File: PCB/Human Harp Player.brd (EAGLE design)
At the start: 70 x 70 mm, 41 parts, among them J1 4UCON 20404, J3 Sparkfun: PRT-00553, J4 Sparkfun: PRT-00553, J5 Sparkfun: PRT-00553, J6 Sparkfun: PRT-00553, J7 ICSP, J8 Molex: 500075-1517, Q1 MMBT2222A, Q3 STD26P3LLH6, U1 DSPIC33EP512GM604-I/PT, U2 MIC5319-3.3YD5, U3 Sparkfun: PRT-00116, X1 ABM8-16.000MHZ-B2-T

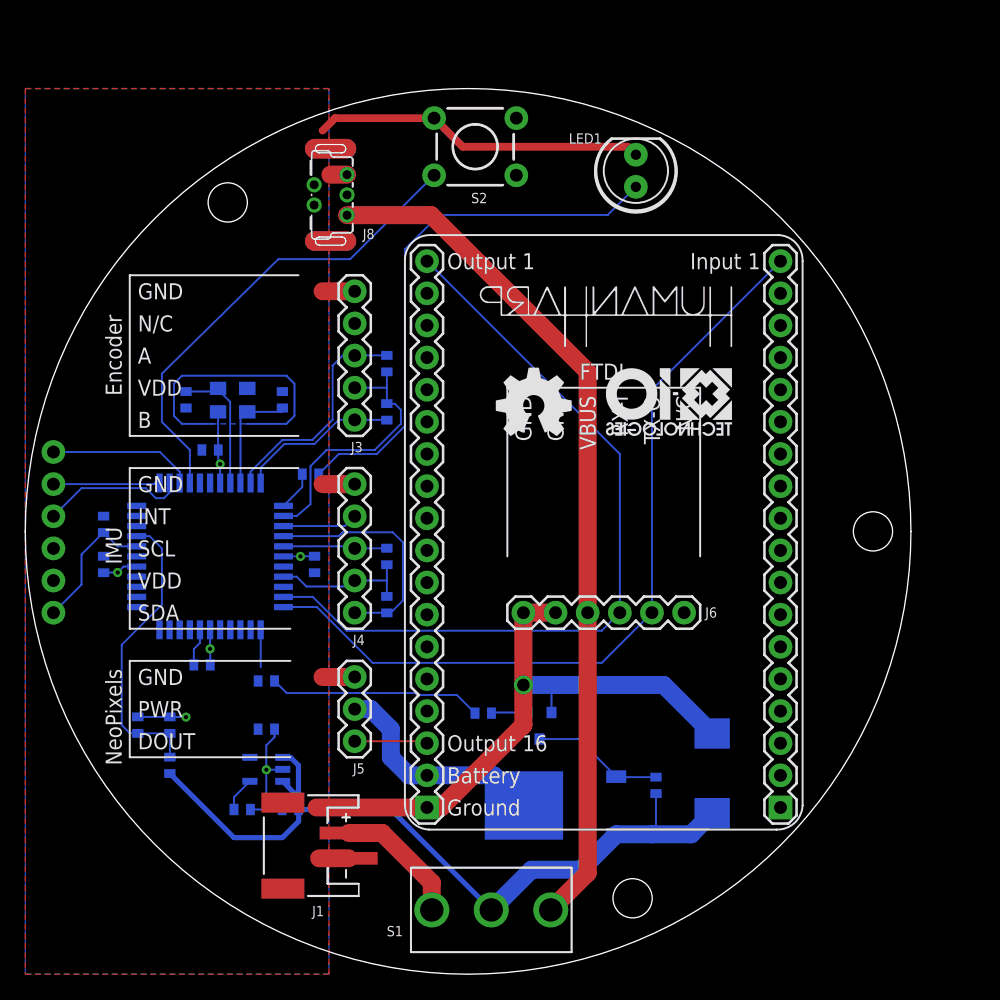
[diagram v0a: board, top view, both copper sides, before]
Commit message: Commit PCB Rev. 2
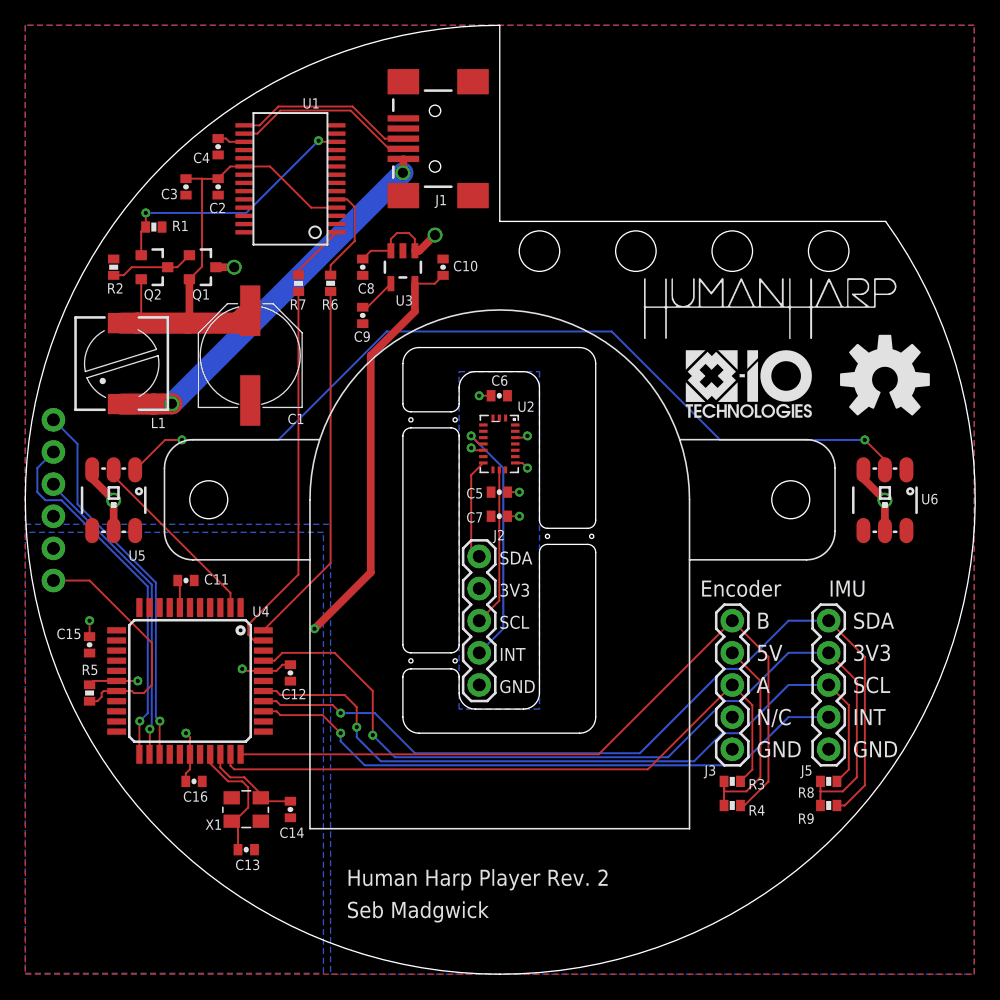
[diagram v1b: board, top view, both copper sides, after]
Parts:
- removed J6: Sparkfun: PRT-00553, SparkFun:1X06
- removed J7: ICSP, SparkFun-Connectors:1X06_NO_SILK
- removed J8: Molex: 500075-1517, x-io:500075-1517
- removed LED1: Sparkfun: COM-12903 (purple), SparkFun-LED:LED5MM
- removed Q3: STD26P3LLH6, transistor-fet:TO252
- removed R10: 10k, 0603, SparkFun:0402-RES
- removed R11: 15R, 0603, SparkFun:0402-RES
- removed S1: RS: 5MS1S102AM2QES, x-io:5MS1S102AM2QES
- removed S2: TE Connectivity: FSM4JAH, SparkFun-Electromechanical:TACTILE-PTH
- removed U$3: (no value), x-io:HUMAN_HARP_LOGO_20MM_BOTTOM
- added C12, C15, C16: 100n, 0603, SparkFun:0402-CAP
- added C13, C14: 22p, 0603, SparkFun:0402-CAP
- added J2: Unpopulated, SparkFun-Connectors:1X05
- added L1: 220u, 510mA, EATON-DRA73-221-R, rcl:PIS2816
- added LOGO1: OSHW-LOGOL, SparkFun-Aesthetics:OSHW-LOGO-L
- added Q2: IRLML6401PBF, SparkFun-DiscreteSemi:SOT23-3
- added U$2: (no value), x-io:HEDS-5600-A06
- added U4: DSPIC33EP512GM604-I/PT, x-io:TQFP44
- added U5, U6: WS2811, SparkFun-LED:LED-TRICOLOR-5050-IC
- C1: value 100n, 0603 -> 470u, 16V, Pansonic F; device SparkFun:0402-CAP -> rcl:PANASONIC_F
- C10, C8: value 100n, 0603 -> 10u, 0603
- C11: value 470u, 10V, Tant, Case E -> 10u, 0603; device rcl:SMC_E -> SparkFun:0402-CAP
- C5, C6: value 22p, 0603 -> 100n, 0603
- C9: value 10u, 0603 -> 100n, 0603
- J1: value 4UCON 20404 -> Sparkfun-PRT-00587; device x-io:JST-R/A -> SparkFun-Connectors:USB-MINIB
- J3: value Sparkfun: PRT-00553 -> Sparkfun: PRT-00116
- J4: value Sparkfun: PRT-00553 -> Unpopulated; device SparkFun-Connectors:1X05 -> SparkFun-Connectors:1X06_NO_SILK
- J5: value Sparkfun: PRT-00553 -> Sparkfun: PRT-00116; device SparkFun-Connectors:1X03 -> SparkFun-Connectors:1X05
- Q1: value MMBT2222A -> IRLML6401PBF
- R1, R6, R7: value 10k 0603 -> 4k7, 0603
- R2, R3, R4, R5, R8, R9: value 10k, 0603 -> 4k7, 0603
- U$1: device x-io:X-IO_TECHNOLOGIES_LOGO_10MM_BOTTOM -> x-io:X-IO_TECHNOLOGIES_LOGO_10MM_TOP
- U$4: value OSHW_LOGO6MM_BOTTOM -> (none); device x-io:OSHW_LOGO_6MM_BOTTOM -> x-io:HUMAN_HARP_LOGO_20MM_TOP
- U1: value DSPIC33EP512GM604-I/PT -> FT232RL; device x-io:TQFP44 -> SparkFun:SSOP28DB
- U2: value MIC5319-3.3YD5 -> BMX055; device x-io:SOT23-5 -> x-io:BMX055
- U3: value Sparkfun: PRT-00116 -> MIC5319-3.3YD5; device x-io-EAGLE-Library:X-OSC_TH -> x-io:SOT23-5
- X1: value ABM8-16.000MHZ-B2-T -> ABRACON-ABM8-16.000MHZ-B2-T
- moved J1 56.9 mm to (32.4, 66.0), turned to 180 degrees
- moved R8 45.2 mm to (63.5, 15.2), flipped to the top, turned to 180 degrees
- moved Q1 45.0 mm to (14.0, 55.9), flipped to the top, turned to 270 degrees
- moved C11 44.3 mm to (12.7, 31.1), flipped to the top, turned to 0 degrees
- moved C8 43.9 mm to (26.7, 55.9), flipped to the top, turned to 270 degrees
- moved C10 43.5 mm to (33.0, 55.9), flipped to the top
- moved R6 40.2 mm to (24.1, 54.6), flipped to the top
- moved R3 40.0 mm to (55.9, 15.2), flipped to the top, turned to 180 degrees
- moved C2 37.8 mm to (15.2, 62.2), flipped to the top, turned to 90 degrees
- moved J5 37.7 mm to (63.5, 27.9)
- moved R7 36.4 mm to (21.6, 54.6), flipped to the top
- moved J3 33.8 mm to (55.9, 27.9), turned to 270 degrees
- moved R4 33.7 mm to (55.9, 13.3), flipped to the top, turned to 180 degrees
- moved C9 33.6 mm to (26.7, 52.1), flipped to the top, turned to 270 degrees
- moved U2 31.6 mm to (37.5, 41.9), flipped to the top, turned to 0 degrees
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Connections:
- removed net AUX: J7.6, U1.25
- removed net BATTERY_LEVEL: C10.1, R6.1, R7.2, U1.19
- removed net BUTTON: S2.3, U1.26
- removed net ENCODER_VDD: J3.2, R2.2, R3.2, U1.35
- removed net IMU_INT: J4.4, U1.36
- removed net IMU_SCL: J4.3, R4.1, U1.38
- removed net IMU_SDA: J4.1, R5.1, U1.37
- removed net IMU_VDD: J4.2, R4.2, R5.2, U1.41
- removed net IN1: J6.2, U1.44, U3.1
- removed net LED: R11.1, U1.34
- removed net OUT1: J6.3, U1.43, U3.36
- removed net OUT16: J5.3, U3.21
- removed net POWER_ENABLE: U1.1
- removed net VIN: C11.+, C7.1, Q3.2, R6.2, R9.2, S1.2, U2.1, U2.3
- removed net X-OSC_ENABLE: R10.2, R8.1
- removed net X-OSC_PWR: J5.2, Q3.3, U3.20
- new net 3V3: C10.1, C12.1, C15.1, C16.2, R5.1, U3.5, U4.17, U4.28, U4.40
- new net 5V: C8.1, J3.2, Q1.3, R3.2, R4.2, U3.1, U3.3, U5.3, U5.5, U6.3, U6.5
- new net BMX055_INT: J2.4, J5.4, U2.14, U4.36
- new net BMX055_SCL: J2.3, J5.3, R8.1, U2.9, U4.38
- new net BMX055_SDA: J2.1, J5.1, R9.1, U2.11, U4.37
- new net FTDI_D+: J1.D+, U1.15
- new net FTDI_D-: J1.D-, U1.16
- new net FTDI_RX: R6.1, U1.5
- new net FTDI_SLEEP: Q2.1, R1.2, U1.12
- new net FTDI_TX: R7.1, U1.1
- new net N$6: J1.VBUS, L1.1
- new net N$8: U5.1, U6.2
- new net TEST: J4.6, U4.25
- new net VSENSORS: C5.1, C6.1, C7.2, J2.2, J5.2, R8.2, R9.2, U2.13, U2.3, U2.7, U4.41
- new net WS2811_DATA: U4.2, U5.2
- net ENCODER_A: now also R3.1, U4.32; no longer R2.1, U1.32
- net ENCODER_B: now also R4.1, U4.33; no longer R3.1, U1.33
- net GND: now also C1.-, C11.2, C12.2, C13.1, C14.1, C15.2, C16.1, C2.1, C3.1, C7.1, J1.GND, J2.5, J4.3, J5.5, R1.1, R2.1, U1.11, U1.18, U1.21, U1.25, U1.26, U1.7, U2.12, U2.17, U2.20, U2.4, U2.6, U3.2, U4.16, U4.29, U4.39, U4.6, U5.6, U6.6; no longer C1.2, C11.-, C2.2, C3.2, C7.2, J1.-, J4.5, J5.1, J6.5, J6.6, J7.3, J8.GND, LED1.K, Q1.2, R7.1, S2.1, U1.16, U1.29, U1.39, U1.6, U2.2, U3.19
- net MCLR: now also J4.1, R5.2, U4.18; no longer J7.1, R1.2, U1.18
- net N$1: now also Q2.3, R2.2; no longer R10.1
- net N$2: now also R6.2, U4.44; no longer J1.+, S1.3
- net N$3: now also C4.2, U1.17; no longer LED1.A, R11.2
- net N$4: now also C11.1, U4.7; no longer C2.1, U1.7
- net N$5: now also R7.2, U4.43; no longer Q1.3, Q3.1, R9.1
- net N$7: now also C9.1, U3.4; no longer C8.1, U2.4
- net OSC1: now also C13.2, U4.30, X1.3; no longer C6.1, U1.30, X1.1
- net OSC2: now also C14.2, U4.31, X1.1; no longer C5.1, U1.31, X1.3
- net PGEC1: now also J4.5, U4.23; no longer J7.5, U1.23
- net PGED1: now also J4.4, U4.24; no longer J7.4, U1.24
- net VBUS: now also C1.+, C2.2, C3.2, L1.2, Q1.2, Q2.2, U1.20, U1.4; no longer J6.4, J8.VBUS, S1.1
- net VDD: now also J4.2; no longer C1.1, C3.1, C4.2, C9.1, J7.2, R1.1, R8.2, U1.17, U1.28, U1.40, U2.5
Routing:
- net GND: track 138.3 -> 0.00 mm, vias 7 -> 0
- net BMX055_SDA: track 0.00 -> 75.8 mm, vias 0 -> 1
- net VSENSORS: track 0.00 -> 75.8 mm, vias 0 -> 7
- net BMX055_SCL: track 0.00 -> 72.1 mm, vias 0 -> 1
- net N$8: track 0.00 -> 68.8 mm, vias 0 -> 2
- net BMX055_INT: track 0.00 -> 68.6 mm, vias 0 -> 2
- net IN1: track 64.6 -> 0.00 mm
- net VIN: track 63.0 -> 0.00 mm
- net OUT1: track 62.4 -> 0.00 mm
- net ENCODER_B: track 12.8 -> 60.1 mm
- net 3V3: track 0.00 -> 46.4 mm, vias 0 -> 5
- net N$3: track 42.7 -> 2.17 mm
- net 5V: track 0.00 -> 38.0 mm, vias 0 -> 4
- net BUTTON: track 37.5 -> 0.00 mm
- net ENCODER_A: track 18.0 -> 52.1 mm
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- added copper zone on layer 16, net 3V3
- added copper zone on layer 16, net 5V
- added copper zone on layer 16, net VSENSORS
- removed copper zone on layer 16, net GND
- removed copper zone on layer 16, net VDD
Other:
- board size 70 x 70 mm -> 75.1 x 75 mm
- board text added: "3V3"
- board text added: "5V"
- board text added: "Human Harp Player Rev. 2"
- board text added: "TEST"
- board text removed: "AUX"
- board text removed: "Battery"
- board text removed: "DOUT"
- board text removed: "FTDI"
- board text removed: "Ground"
- board text removed: "Human Harp Player v1.0"
- board text removed: "Input 1"
- board text removed: "NeoPixels"
- board text removed: "Output 1"
- board text removed: "Output 16"
- board text removed: "PWR"
- board text removed: "RX-I"
- board text removed: "TX-O"
- board text removed: "VBUS"
